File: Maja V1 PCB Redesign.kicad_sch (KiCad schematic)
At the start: 21 parts, among them J1 TYPE-C-31-M-12, J2 AVR-ISP-6, U1 ATmega32U4-M, U2 PRTR5V0U2X, Y1 Crystal_GND24_Small

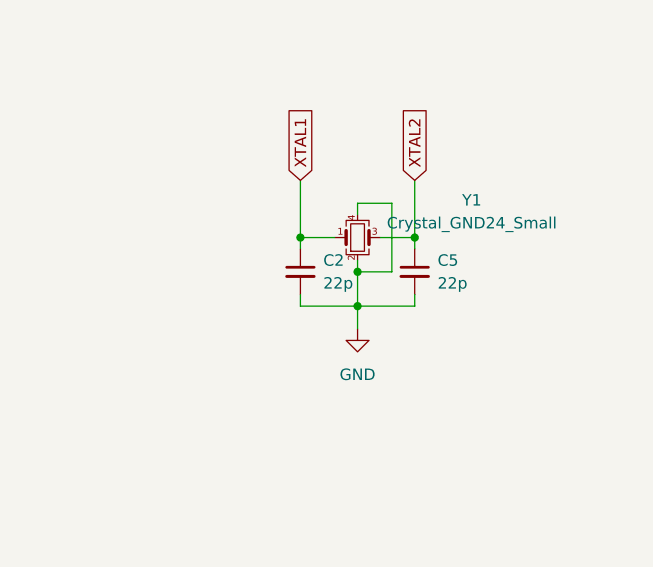
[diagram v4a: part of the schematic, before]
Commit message: LCSC Component
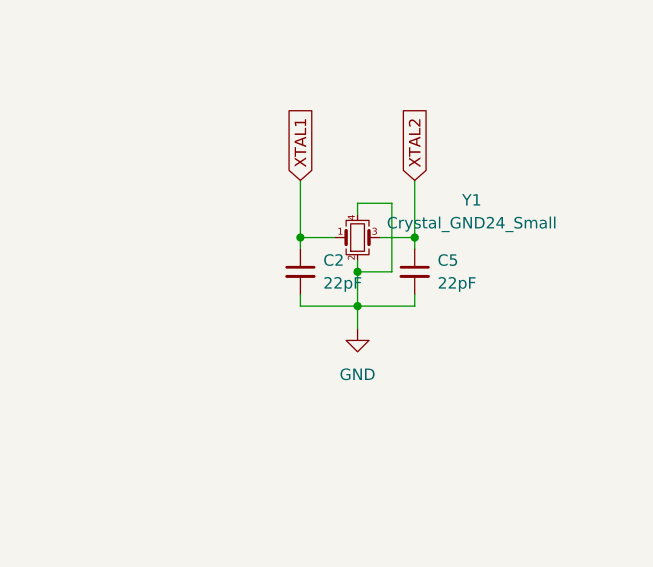
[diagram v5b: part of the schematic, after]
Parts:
- C1: LCSC (none) -> C116352
- C2, C5: value 22p -> 22pF; LCSC (none) -> C1804
- C3, C4, C6, C7: LCSC (none) -> C1760
- C8: LCSC (none) -> C95841
- F1: LCSC (none) -> C70069
- J1: LCSC (none) -> C165948
- R1, R2: LCSC (none) -> C84375
- R3, R6: LCSC (none) -> C84376
- R4, R5: LCSC (none) -> C150390
- S1: LCSC (none) -> C202424
- U2: LCSC (none) -> C12333
- Y1: LCSC (none) -> C12668
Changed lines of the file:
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@@
       (effects (font (size 1.27 1.27)) (justify left))
     )
-    (property "Value" "22p" (id 1) (at 250.19 93.9862 0)
+    (property "Value" "22pF" (id 1) (at 250.19 93.9862 0)
       (effects (font (size 1.27 1.27)) (justify left))
     )
@@
       (effects (font (size 1.27 1.27)) hide)
     )
+    (property "LCSC" "C1804" (id 4) (at 247.65 92.71 0)
+      (effects (font (size 1.27 1.27)) hide)
+    )
     (pin "1")
     (pin "2")
@@
     )
     (property "Datasheet" "~" (id 3) (at 64.77 109.22 0)
+      (effects (font (size 1.27 1.27)) hide)
+    )
+    (property "LCSC" "C84375" (id 4) (at 64.77 109.22 0)
       (effects (font (size 1.27 1.27)) hide)
     )
@@
       (effects (font (size 1.27 1.27)) hide)
     )
+    (property "LCSC" "C84376" (id 4) (at 182.88 111.76 90)
+      (effects (font (size 1.27 1.27)) hide)
+    )
     (pin "1")
     (pin "2")
@@
     (property "STANDARD" "Manufacturer Recommendations" (id 7) (at 63.5 64.77 0)
       (effects (font (size 1.27 1.27)) (justify left bottom) hide)
+    )
+    (property "LCSC" "C165948" (id 8) (at 35.56 90.17 0)
+      (effects (font (size 1.27 1.27)) hide)
     )
     (pin "A1B12")
@@
       (effects (font (size 1.27 1.27)) hide)
     )
+    (property "LCSC" "C1760" (id 4) (at 257.81 139.7 0)
+      (effects (font (size 1.27 1.27)) hide)
+    )
     (pin "1")
     (pin "2")
@@
       (effects (font (size 1.27 1.27)) hide)
     )
+    (property "LCSC" "C150390" (id 4) (at 105.41 99.06 90)
+      (effects (font (size 1.27 1.27)) hide)
+    )
     (pin "1")
     (pin "2")
@@
     )
     (property "Datasheet" "~" (id 3) (at 137.16 93.98 0)
+      (effects (font (size 1.27 1.27)) hide)
+    )
+    (property "LCSC" "C116352" (id 4) (at 137.16 93.98 0)
       (effects (font (size 1.27 1.27)) hide)
     )
@@
     )
     (property "Datasheet" "~" (id 3) (at 264.16 139.7 0)
+      (effects (font (size 1.27 1.27)) hide)
+    )
+    (property "LCSC" "C95841" (id 4) (at 264.16 139.7 0)
       (effects (font (size 1.27 1.27)) hide)
     )
@@
       (effects (font (size 1.27 1.27)) hide)
     )
+    (property "LCSC" "C70069" (id 4) (at 69.85 86.36 90)
+      (effects (font (size 1.27 1.27)) hide)
+    )
     (pin "1")
     (pin "2")
@@
       (effects (font (size 1.27 1.27)) (justify left))
     )
-    (property "Value" "22p" (id 1) (at 237.49 93.9862 0)
+    (property "Value" "22pF" (id 1) (at 237.49 93.9862 0)
       (effects (font (size 1.27 1.27)) (justify left))
     )
@@
     )
     (property "Datasheet" "~" (id 3) (at 234.95 92.71 0)
+      (effects (font (size 1.27 1.27)) hide)
+    )
+    (property "LCSC" "C1804" (id 4) (at 234.95 92.71 0)
       (effects (font (size 1.27 1.27)) hide)
     )
@@
       (effects (font (size 1.27 1.27)) (justify left bottom) hide)
     )
+    (property "LCSC" "C202424" (id 7) (at 71.12 36.83 0)
+      (effects (font (size 1.27 1.27)) hide)
+    )
     (pin "1")
     (pin "2")
@@
       (effects (font (size 1.27 1.27)) hide)
     )
-    (property "Datasheet" "~" (id 3) (at 242.57 139.7 0)
+    (property "Datasheet" "~" (id 3) (at 242.57 139.7 0))
+    (property "LCSC" "C1760" (id 4) (at 242.57 139.7 0)
       (effects (font (size 1.27 1.27)) hide)
     )
@@
     (property "Datasheet" "" (id 3) (at 92.71 109.22 0)
       (effects (font (size 1.524 1.524)) hide)
+    )
+    (property "LCSC" "C12333" (id 4) (at 92.71 109.22 0)
+      (effects (font (size 1.27 1.27)) hide)
     )
     (pin "1")
@@
       (effects (font (size 1.27 1.27)) hide)
     )
+    (property "LCSC" "C12668" (id 4) (at 241.3 88.9 0)
+      (effects (font (size 1.27 1.27)) hide)
+    )
     (pin "1")
     (pin "2")
@@
       (effects (font (size 1.27 1.27)) hide)
     )
+    (property "LCSC" "C84375" (id 4) (at 73.66 109.22 0)
+      (effects (font (size 1.27 1.27)) hide)
+    )
     (pin "1")
     (pin "2")
@@
       (effects (font (size 1.27 1.27)) hide)
     )
+    (property "LCSC" "C1760" (id 4) (at 234.95 139.7 0)
+      (effects (font (size 1.27 1.27)) hide)
+    )
     (pin "1")
     (pin "2")
@@
     )
     (property "Datasheet" "~" (id 3) (at 82.55 29.21 0)
+      (effects (font (size 1.27 1.27)) hide)
+    )
+    (property "LCSC" "C84376" (id 4) (at 82.55 29.21 0)
       (effects (font (size 1.27 1.27)) hide)
     )
@@
     )
     (property "Datasheet" "~" (id 3) (at 250.19 139.7 0)
+      (effects (font (size 1.27 1.27)) hide)
+    )
+    (property "LCSC" "C1760" (id 4) (at 250.19 139.7 0)
       (effects (font (size 1.27 1.27)) hide)
     )
@@
       (effects (font (size 1.27 1.27)) hide)
     )
+    (property "LCSC" "C150390" (id 4) (at 105.41 101.6 90)
+      (effects (font (size 1.27 1.27)) hide)
+    )
     (pin "1")
     (pin "2")
@@
     )
     (path "/805d97db-8b85-4718-87ad-38794fb3e6e5"
-      (reference "C2") (unit 1) (value "22p") (footprint "Capacitor_SMD:C_0805_2012Metric_Pad1.18x1.45mm_HandSolder")
+      (reference "C2") (unit 1) (value "22pF") (footprint "Capacitor_SMD:C_0805_2012Metric_Pad1.18x1.45mm_HandSolder")
     )
     (path "/c21145b3-2ba8-4199-bd62-8a52576b0f76"
@@
     )
     (path "/1276ab35-37a9-4274-924a-3f362baae999"
-      (reference "C5") (unit 1) (value "22p") (footprint "Capacitor_SMD:C_0805_2012Metric_Pad1.18x1.45mm_HandSolder")
+      (reference "C5") (unit 1) (value "22pF") (footprint "Capacitor_SMD:C_0805_2012Metric_Pad1.18x1.45mm_HandSolder")
     )
     (path "/e770da12-986a-45ad-a103-4032138ba68c"
